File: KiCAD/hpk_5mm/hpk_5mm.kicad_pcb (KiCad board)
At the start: 2 copper layers, 7.4 x 7.4 mm, 4 parts, among them J1 Conn_01x03

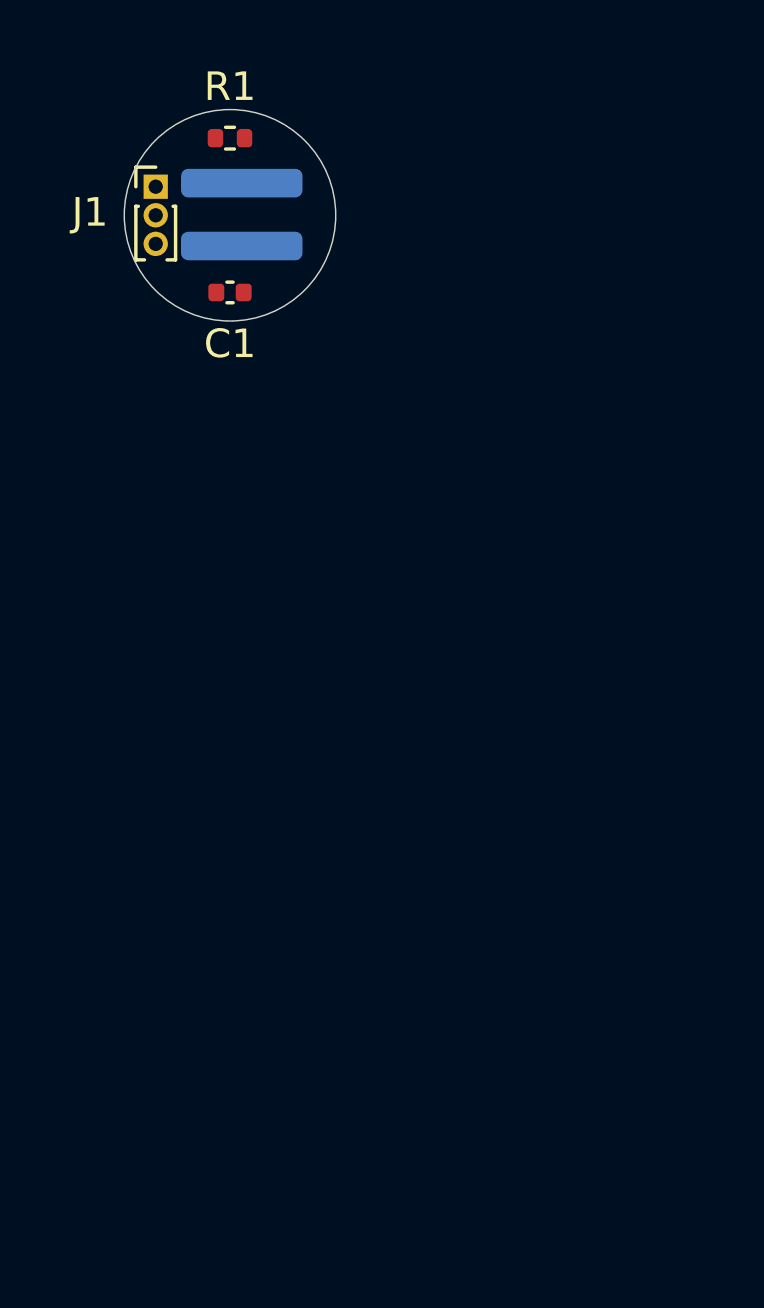
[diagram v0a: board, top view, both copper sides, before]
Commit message: trial 3-channel flexi
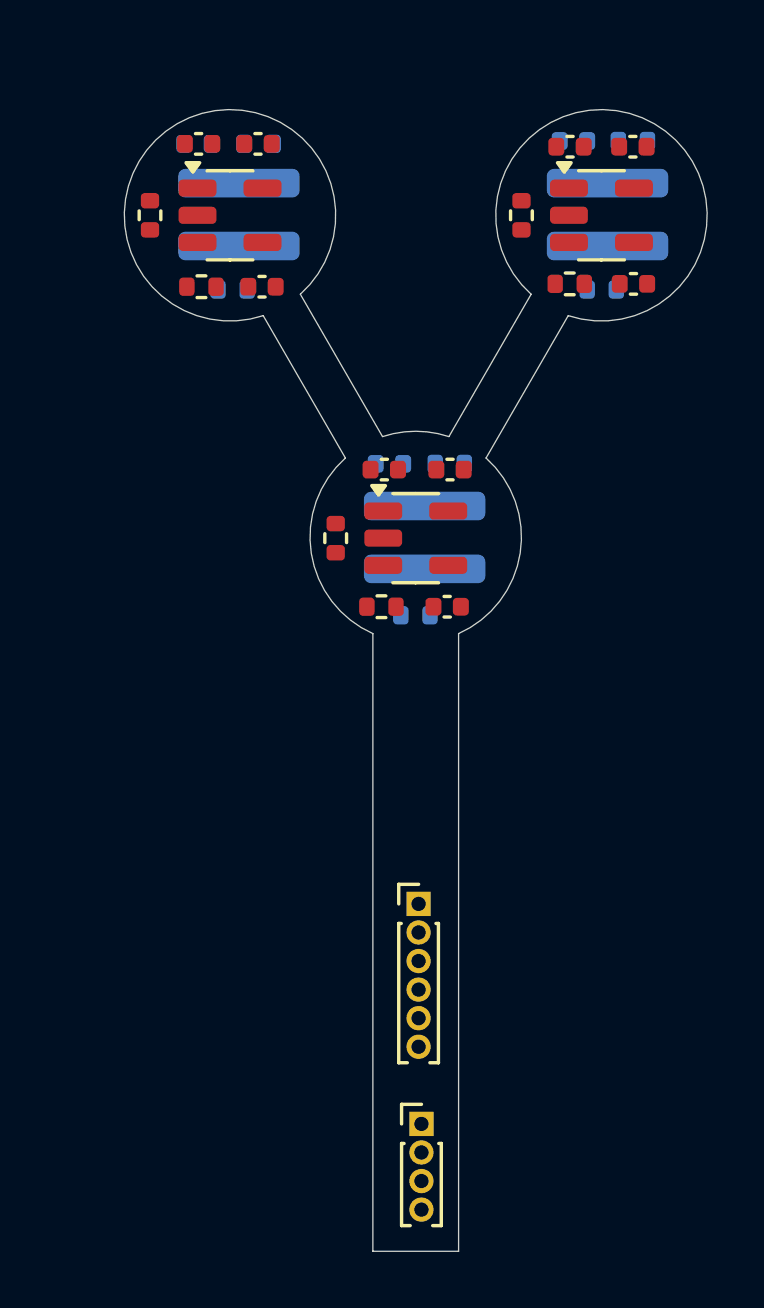
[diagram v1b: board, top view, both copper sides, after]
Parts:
- added C10: 0.1uF, Capacitor_SMD:C_0402_1005Metric, F.Cu at (147.7, 78.9)
- added C11: 0.1uF, Capacitor_SMD:C_0402_1005Metric, F.Cu at (147.6, 83.7)
- added C12: 0.1uF, Capacitor_SMD:C_0402_1005Metric, F.Cu at (145.4, 78.9)
- added C2: 0.1uF, Capacitor_SMD:C_0402_1005Metric, F.Cu at (141.0, 67.5)
- added C3: 0.1uF, Capacitor_SMD:C_0402_1005Metric, F.Cu at (141.1, 72.5)
- added C4: 0.1uF, Capacitor_SMD:C_0402_1005Metric, F.Cu at (138.9, 67.5)
- added C5: 0.1uF, Capacitor_SMD:C_0402_1005Metric, B.Cu at (152.0, 67.4)
- added C6: 0.1uF, Capacitor_SMD:C_0402_1005Metric, F.Cu at (154.1, 67.6)
- added C7: 0.1uF, Capacitor_SMD:C_0402_1005Metric, F.Cu at (154.1, 72.4)
- added C8: 0.1uF, Capacitor_SMD:C_0402_1005Metric, F.Cu at (151.9, 67.6)
- added C9: 0.1uF, Capacitor_SMD:C_0402_1005Metric, B.Cu at (145.6, 78.7)
- added D2: S13360-3050PE, my_sipm:s13360-3050pe, B.Cu at (153.2, 68.9)
- added D3: S13360-3050PE, my_sipm:s13360-3050pe, B.Cu at (146.8, 80.2)
- added J2: Conn_01x06, Connector_PinHeader_1.00mm:PinHeader_1x06_P1.00mm_Vertical, F.Cu at (146.6, 94.1)
- added R10: 1k, Resistor_SMD:R_0402_1005Metric, B.Cu at (146.5, 84.0)
- added R11: 1k, Resistor_SMD:R_0402_1005Metric, F.Cu at (145.3, 83.7)
- added R12: 1k, Resistor_SMD:R_0402_1005Metric, F.Cu at (143.7, 81.3)
- added R2: 1k, Resistor_SMD:R_0402_1005Metric, B.Cu at (140.1, 72.6)
- added R3: 1k, Resistor_SMD:R_0402_1005Metric, F.Cu at (139.0, 72.5)
- added R4: 1k, Resistor_SMD:R_0402_1005Metric, F.Cu at (137.2, 70.0)
- added R5: 1k, Resistor_SMD:R_0402_1005Metric, B.Cu at (154.1, 67.4)
- added R6: 1k, Resistor_SMD:R_0402_1005Metric, B.Cu at (153.0, 72.6)
- added R7: 1k, Resistor_SMD:R_0402_1005Metric, F.Cu at (151.9, 72.4)
- added R8: 1k, Resistor_SMD:R_0402_1005Metric, F.Cu at (150.2, 70.0)
- added R9: 1k, Resistor_SMD:R_0402_1005Metric, B.Cu at (147.7, 78.7)
- added U1: OPA810xDBV, Package_TO_SOT_SMD:SOT-23-5, F.Cu at (140.0, 70.0)
- added U2: OPA810xDBV, Package_TO_SOT_SMD:SOT-23-5, F.Cu at (153.0, 70.0)
- added U3: OPA810xDBV, Package_TO_SOT_SMD:SOT-23-5, F.Cu at (146.5, 81.3)
- C1, R1: moved to B.Cu
- J1: value Conn_01x03 -> Conn_01x04; footprint Connector_PinHeader_1.00mm:PinHeader_1x03_P1.00mm_Vertical -> Connector_PinHeader_1.00mm:PinHeader_1x04_P1.00mm_Vertical
- moved J1 34.1 mm to (146.7, 101.8)
- moved C1 5.32 mm to (138.9, 67.5), turned to 180 degrees
- moved R1 1.02 mm to (141.0, 67.5), turned to 180 degrees
- moved D1 0.10 mm to (140.3, 68.9)
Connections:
- J1 pad 1: Net-(J1-Pin_1) -> /sipm_tia1/V+
- J1 pad 3: Net-(D1-A) -> /sipm_tia1/V-
- R1 pad 1: Net-(J1-Pin_1) -> /sipm_tia1/VBIAS
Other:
- board size 7.4 x 7.4 mm -> 20.4 x 40 mm
